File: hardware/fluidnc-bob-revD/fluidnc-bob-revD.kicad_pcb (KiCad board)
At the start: 2 copper layers, 95 x 129.9 mm, 65 parts, among them J1 5V-IN, J10 SPINDLE-SW, J11 AUX, J13 SD, J2 X-DRV, J3 Y-DRV, J4 Z-DRV, J5 LIM-X, J6 LIM-Y, J7 LIM-Z, J8 PROBE, J9 E-STOP, Q1 MMBT2222A, Q2 MMBT2222A, U1 SN74AHCT541N

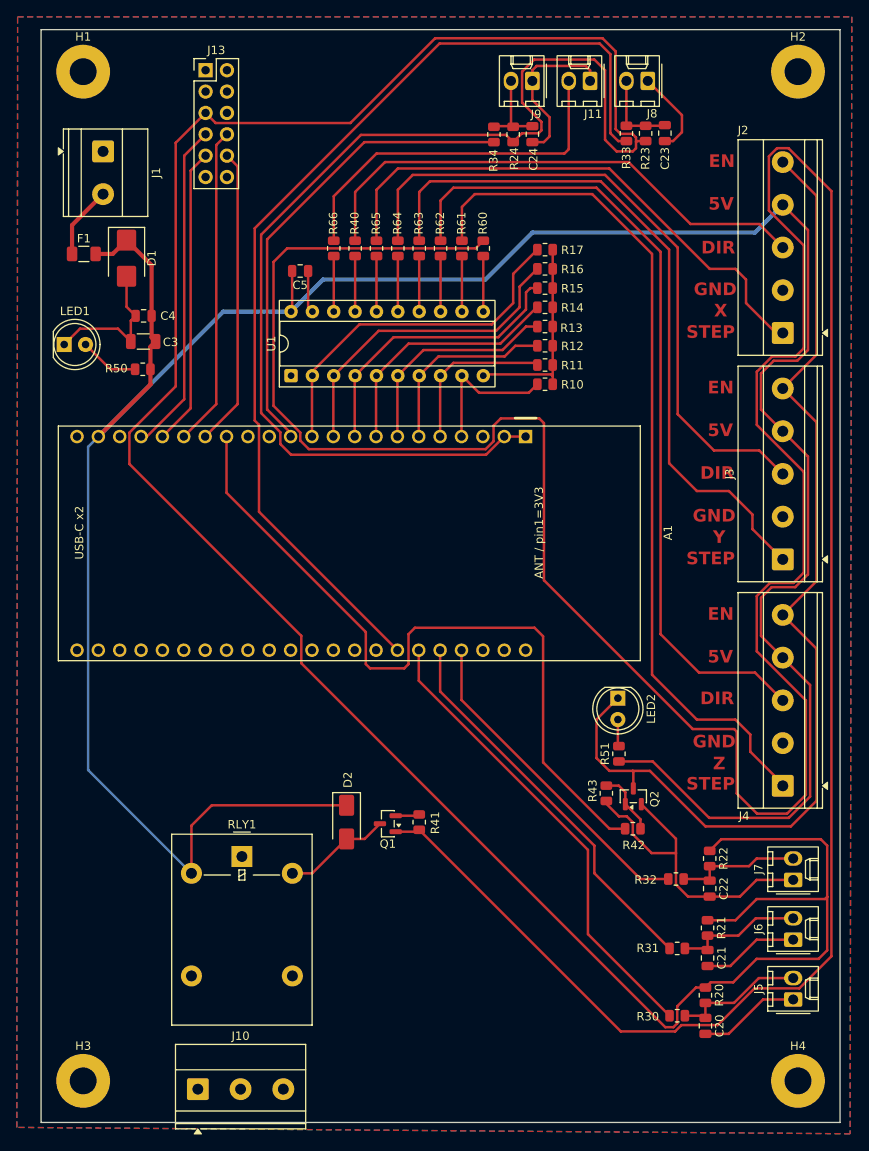
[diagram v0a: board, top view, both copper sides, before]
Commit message: New layout
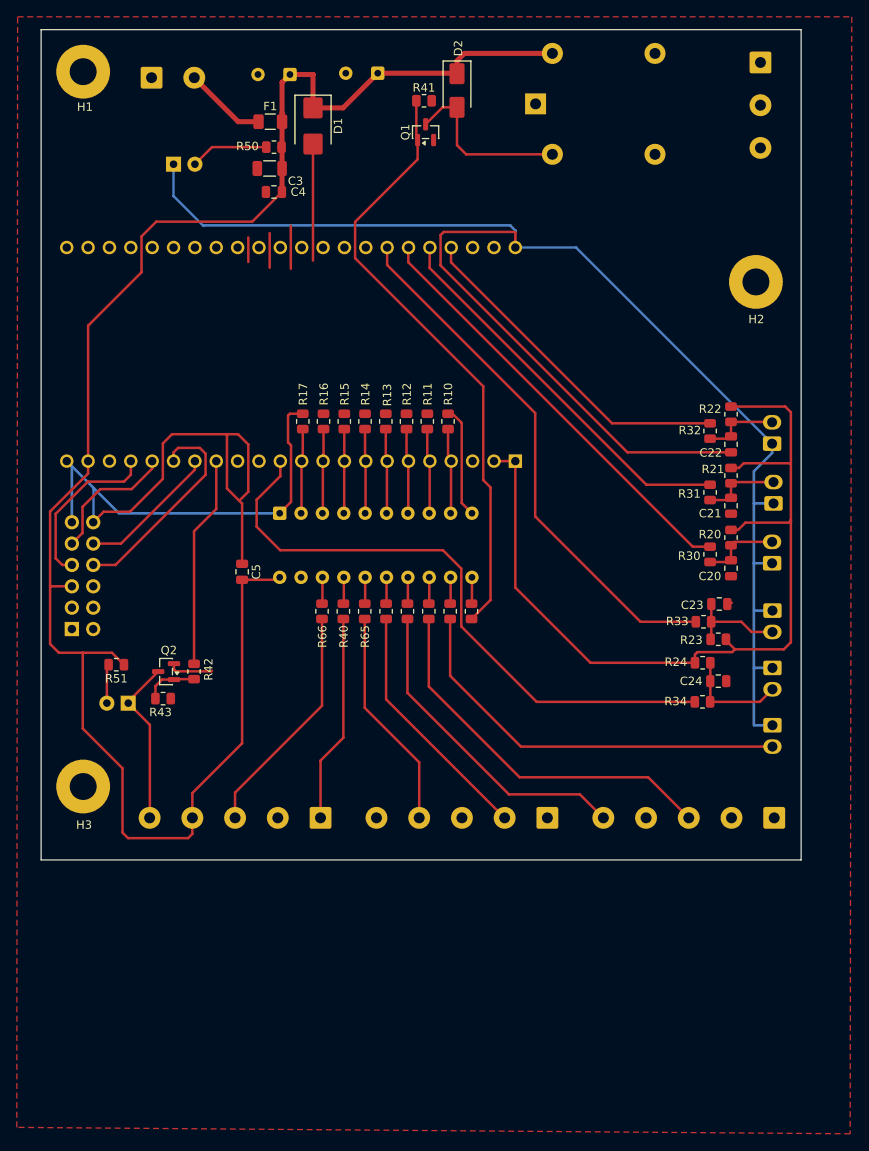
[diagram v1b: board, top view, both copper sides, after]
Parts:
- removed H4: M3, MountingHole:MountingHole_3.2mm_M3_Pad
- added C2: C_Polarized_US, Capacitor_THT:CP_Radial_D8.0mm_P3.80mm, B.Cu at (40.0, 5.18)
- added C6: C_Polarized_US, Capacitor_THT:CP_Radial_D8.0mm_P3.80mm, B.Cu at (29.6, 5.33)
- A1, J1, J11, J13, J5, J6, J7, J8, J9, LED1, LED2, RLY1, U1: moved to B.Cu
- J2: value X-DRV -> EN+X; moved to B.Cu
- J3: value Y-DRV -> X+Y; moved to B.Cu
- J4: value Z-DRV -> Z+5; moved to B.Cu
- SPINDLE: renamed from J10; moved to B.Cu
- moved SPINDLE 139.2 mm to (85.5, 3.91), turned to -90 degrees
- moved RLY1 96.1 mm to (58.8, 8.83), turned to -90 degrees
- moved D2 88.0 mm to (49.5, 7.24)
- moved R41 85.8 mm to (45.5, 8.46), turned to 0 degrees
- moved Q1 82.4 mm to (45.7, 12.2), turned to 90 degrees
- moved J11 79.6 mm to (87.0, 82.7), turned to -90 degrees
- moved J9 75.4 mm to (87.0, 75.9), turned to -90 degrees
- moved R34 71.9 mm to (78.6, 79.9), turned to 0 degrees
- moved C24 68.7 mm to (80.5, 77.5), turned to 0 degrees
- moved J13 68.3 mm to (3.66, 71.3)
- moved R24 66.7 mm to (78.7, 75.3), turned to 0 degrees
- moved J8 64.7 mm to (87.0, 69.1), turned to -90 degrees
- moved R23 60.8 mm to (80.5, 72.5), turned to 180 degrees
- moved R51 60.7 mm to (8.94, 75.5), turned to 180 degrees
- moved R33 58.8 mm to (78.8, 70.4), turned to 0 degrees
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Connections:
- J13 pad 5: +3V3 -> +5V
- J2 pad 1: XSTEP -> unconnected-(J2-Pad1)
- J2 pad 4: +5V -> GND
- J2 pad 5: EN_SINK -> XSTEP
- J3 pad 1: YSTEP -> GND
- J3 pad 2: GND -> YDIR
- J3 pad 3: YDIR -> GND
- J3 pad 4: +5V -> YSTEP
- J3 pad 5: EN_SINK -> GND
- J4 pad 1: ZSTEP -> ZDIR
- J4 pad 3: ZDIR -> ZSTEP
- R40 pad 1: XDIR -> ZDIR
- R61 pad 1: ZSTEP -> AUX
- R62 pad 1: ZDIR -> XDIR
- R63 pad 1: YSTEP -> XSTEP
- R65 pad 1: XSTEP -> YSTEP
- R66 pad 1: AUX -> ZSTEP
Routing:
- net SPIN5: track 404.1 -> 72.4 mm
- net +3V3: track 401.6 -> 107.1 mm
- net GND: track 142.7 -> 339.7 mm
- net +5V: track 323.1 -> 207.4 mm
- net EN_SINK: track 125.3 -> 19.9 mm
- net ZSTEP: track 102.6 -> 27.9 mm
- net ZDIR: track 98.0 -> 24.8 mm
- net EN_G: track 87.8 -> 25.2 mm
- net YSTEP: track 84.1 -> 26.3 mm
- net PROBE_G: track 120.8 -> 63.6 mm
- net YDIR: track 78.9 -> 29.5 mm
- net Net-(A1-GPIO18): track 42.6 -> 10.1 mm
- net Net-(A1-GPIO17): track 38.2 -> 10.1 mm
- net XSTEP: track 65.1 -> 38.2 mm
- net Net-(A1-GPIO16): track 34.4 -> 10.0 mm
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- removed copper zone on B.Cu, net GND
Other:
- board size 95 x 129.9 mm -> 90.4 x 98.7 mm
- board text added: "AUX"
- board text added: "E-STOP"
- board text added: "EN +5V ZSTEP GND ZDIR GND YSTEP GND YDIR GND XSTEP GND XDIR GND"
- board text added: "PROBE"
- board text added: "X_LIM"
- board text added: "Y-LIM"
- board text added: "Z-LIM"
- board text removed: "5V"
- board text removed: "DIR"
- board text removed: "EN"
- board text removed: "GND"
- board text removed: "STEP"
- board text removed: "X"
- board text removed: "Y"
- board text removed: "Z"
